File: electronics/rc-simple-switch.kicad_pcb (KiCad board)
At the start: 2 copper layers, 9 parts, among them K1 CONN_3, K2 CONN_3, P1 CONN_5, Q1 PMV30UN, U1 PIC10F200

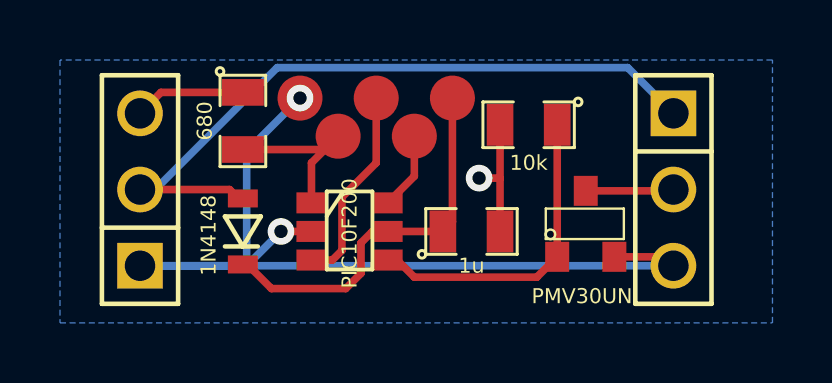
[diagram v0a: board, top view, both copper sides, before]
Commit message: Tweak the PCB
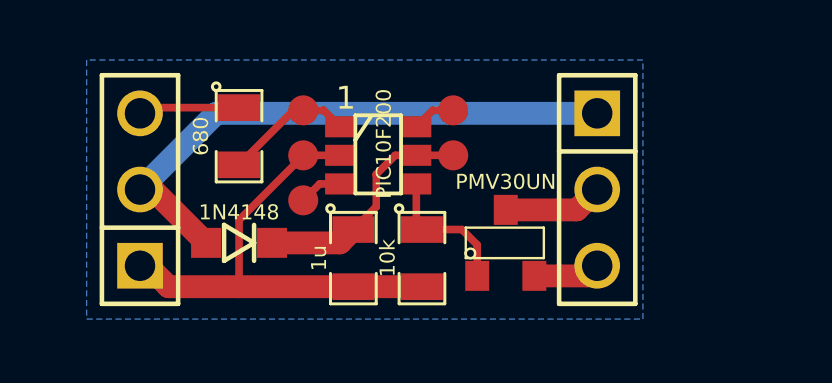
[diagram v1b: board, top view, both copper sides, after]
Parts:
- added P2: CONN_1, Test_pad_1mm, F.Cu at (41.0, 41.0)
- added P3: CONN_1, Test_pad_1mm, F.Cu at (46.0, 38.0)
- added P4: CONN_1, Test_pad_1mm, F.Cu at (41.0, 39.5)
- added P5: CONN_1, Test_pad_1mm, F.Cu at (46.0, 39.5)
- P1: value CONN_5 -> CONN_1; footprint debug_connector -> Test_pad_1mm
- moved R2 5.69 mm to (45.0, 42.9), turned to 270 degrees
- moved C1 4.04 mm to (42.7, 42.9), turned to 270 degrees
- moved Q1 2.74 mm to (47.8, 42.4)
- moved U1 2.71 mm to (43.5, 39.5)
- moved K2 2.54 mm to (50.8, 40.6)
- moved P1 2.47 mm to (41.0, 38.0)
- moved R1 0.52 mm to (38.9, 38.9)
- moved D1 0.40 mm to (38.9, 42.4), turned to 0 degrees
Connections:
- P1 pad 1: VSS -> N-000005
- R1 pad 2: /ICSPDAT -> N-000005
- U1 pad 1: /ICSPDAT -> N-000005
- U1 pad 3: /ICSPCLK -> N-000004
- U1 pad 6: /VPP -> N-000003
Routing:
- net VSS: track 36.6 -> 18.4 mm, vias 3 -> 0
- net /ICSPCLK: track 6.70 -> 0.00 mm
- net /ICSPDAT: track 5.95 -> 0.00 mm
- net /OUT: track 10.6 -> 4.69 mm
- net VDD: track 13.1 -> 7.88 mm
- net VCC: track 23.7 -> 19.2 mm
- net N-000005: track 0.00 -> 4.35 mm
- net /VPP: track 2.59 -> 0.00 mm
- net N-000004: track 0.00 -> 1.46 mm
- net N-000003: track 0.00 -> 1.46 mm
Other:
- net class Power added: clearance 0.508, trace_width 0.254, via_dia 0.889, via_drill 0.635
- board text added: "1"
